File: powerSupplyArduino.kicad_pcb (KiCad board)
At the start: 2 copper layers, 90 x 50 mm, 61 parts, among them J1 supply_shunt, J2 Main connector, J3 Display, J4 Termo_sens, J5 ISP, J6 Encoder, U1 LM324, U2 TL494, U3 ATmega8A-AU

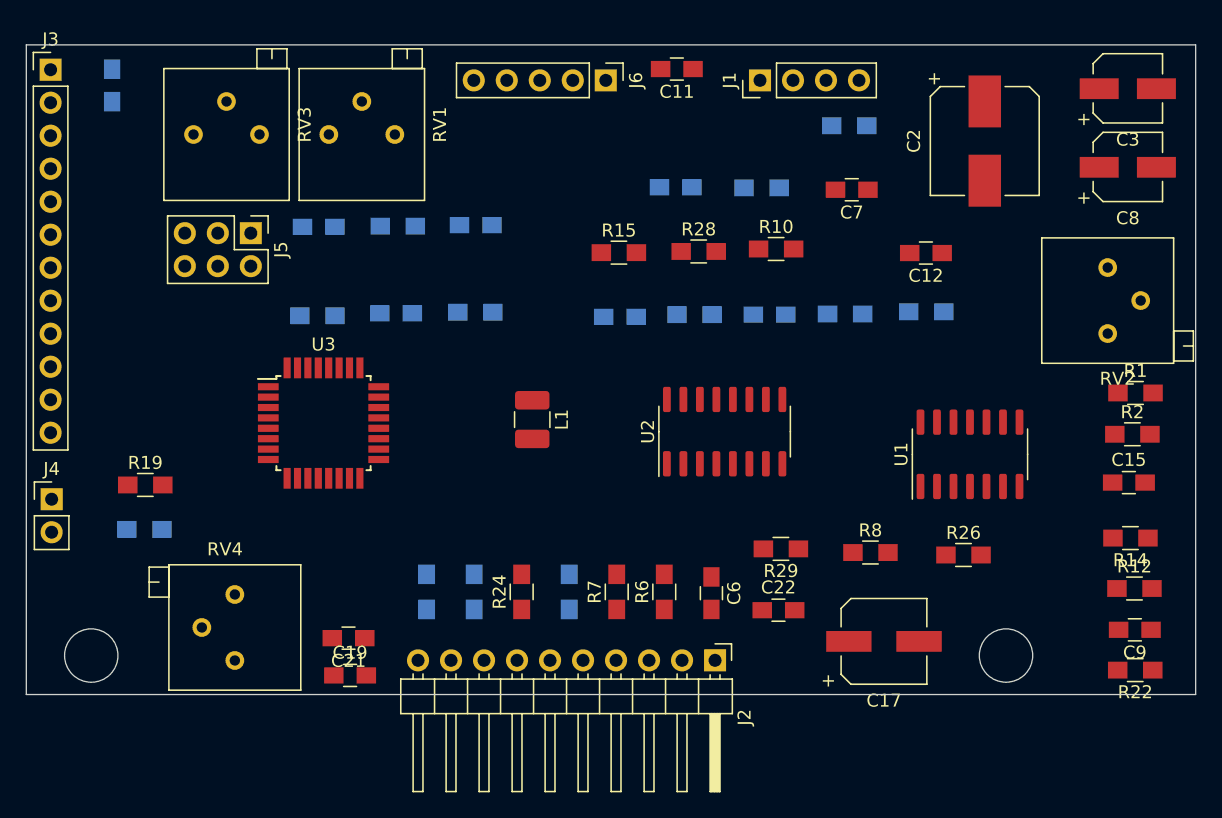
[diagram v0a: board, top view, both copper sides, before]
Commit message: routing complite
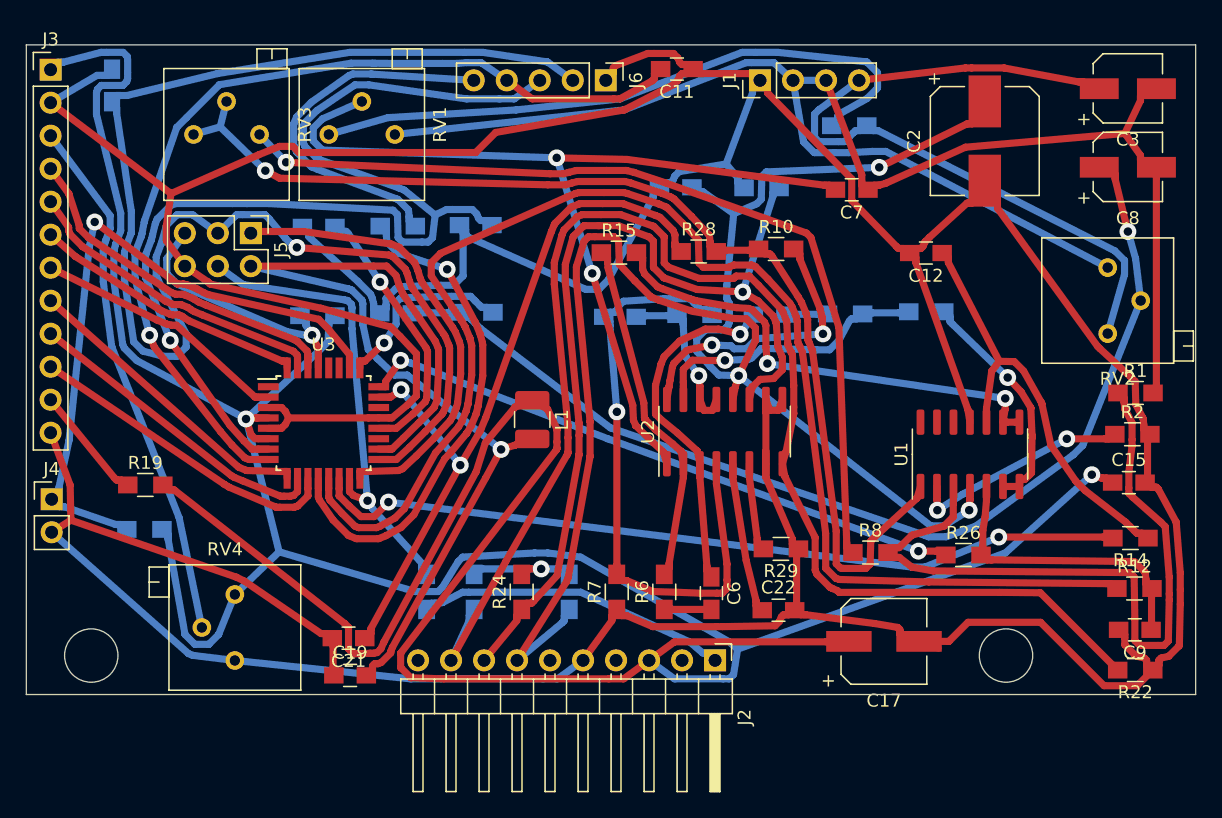
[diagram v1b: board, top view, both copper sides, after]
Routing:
- net GND: track 0.00 -> 415.0 mm
- net +5V: track 0.00 -> 274.9 mm, vias 0 -> 2
- net +15V: track 0.00 -> 129.6 mm, vias 0 -> 3
- net Supply-: track 0.00 -> 120.7 mm
- net Encoder_S: track 0.00 -> 109.9 mm, vias 0 -> 1
- net Q3Base: track 0.00 -> 109.1 mm
- net Net-(R12-Pad1): track 0.00 -> 107.0 mm
- net Net-(R10-Pad1): track 0.00 -> 85.8 mm, vias 0 -> 1
- net Encoder_A: track 0.00 -> 85.2 mm, vias 0 -> 1
- net Net-(C20-Pad1): track 0.00 -> 81.6 mm, vias 0 -> 1
- net ISP_VCC: track 0.00 -> 77.3 mm, vias 0 -> 1
- net Net-(C7-Pad2): track 0.00 -> 71.5 mm, vias 0 -> 2
- net Q4Base: track 0.00 -> 71.1 mm, vias 0 -> 1
- net Encoder_B: track 0.00 -> 71.1 mm, vias 0 -> 1
- net Net-(R8-Pad1): track 0.00 -> 69.2 mm, vias 0 -> 1
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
